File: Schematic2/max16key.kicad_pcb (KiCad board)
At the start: 2 copper layers, 100 x 119 mm, 52 parts, among them SW1 Rotary_Encoder_Switch, U1 Kailhlowprofile, U10 Kailhlowprofile, U11 Kailhlowprofile, U12 Kailhlowprofile, U13 Kailhlowprofile, U14 Kailhlowprofile, U15 Kailhlowprofile, U16 Kailhlowprofile, U17 Kailhlowprofile, U18 Kailhlowprofile, U19 Kailhlowprofile, U2 Kailhlowprofile, U20 Kailhlowprofile, U3 Kailhlowprofile, U4 Kailhlowprofile, U5 Kailhlowprofile, U6 Kailhlowprofile, U7 Kailhlowprofile, U8 Kailhlowprofile, U9 Kailhlowprofile

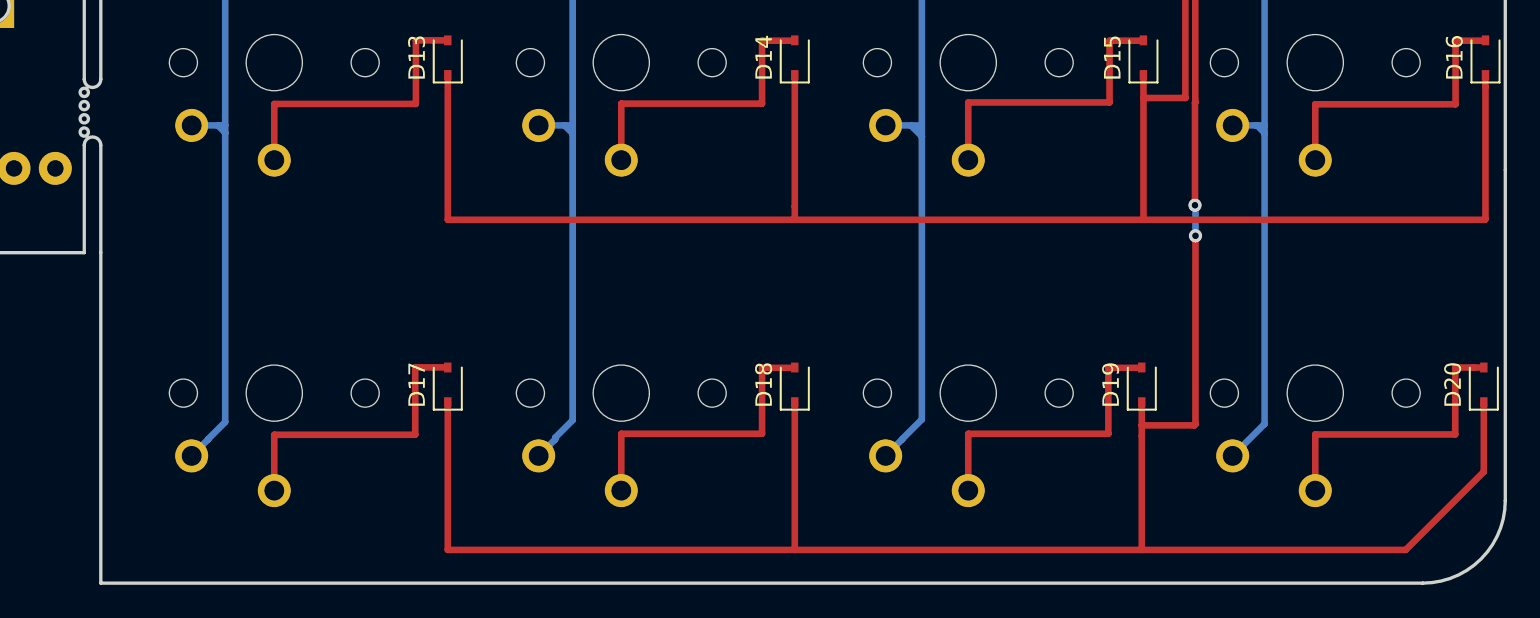
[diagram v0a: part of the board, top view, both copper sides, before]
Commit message: Print time - final and absolutely done edition
This edition is completely done, for realz, and has all the files you need to print a macro keyboard with Kailh switches.
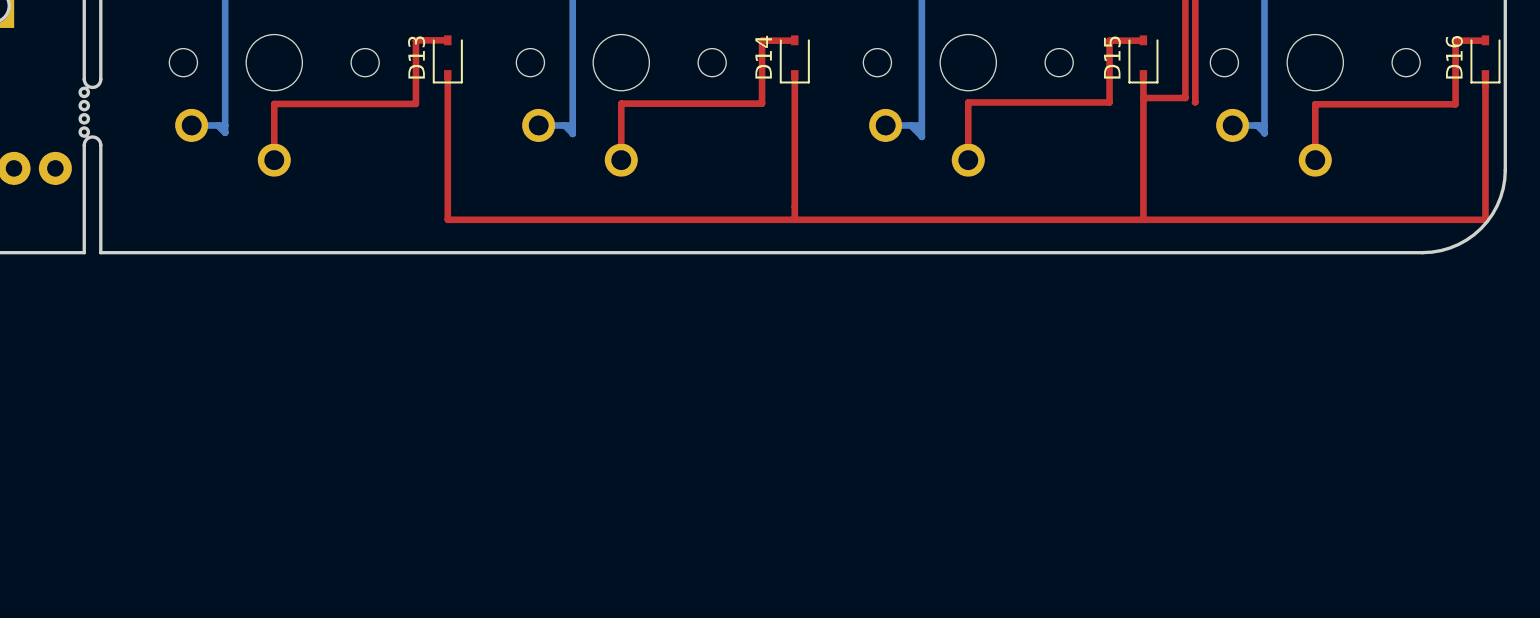
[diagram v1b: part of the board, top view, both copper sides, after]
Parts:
- removed D17, D18, D19, D20: 1N4148WS, Diode_SMD:D_SOD-323
- removed U17, U18, U19, U20: Kailhlowprofile, Keebio-Parts:Kailh-PG1350-1u-No-Clickhole-No-LED
- added G***: LOGO, Schematic2:AI_MF_D12MNeg, B.Cu at (87.0, 95.0)
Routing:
- net R5: track 183.0 -> 64.6 mm, vias 7 -> 5
- net C1: track 159.8 -> 139.4 mm
- net C2: track 141.6 -> 121.3 mm
- net C4: track 109.1 -> 88.8 mm
- net C3: track 123.8 -> 103.6 mm
- net Net-(D17-Pad2): track 18.0 -> 0.00 mm
- net Net-(D19-Pad2): track 17.9 -> 0.00 mm
- net Net-(D18-Pad2): track 17.9 -> 0.00 mm
- net Net-(D20-Pad2): track 17.6 -> 0.00 mm
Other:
- board size 100 x 119 mm -> 100 x 99 mm
